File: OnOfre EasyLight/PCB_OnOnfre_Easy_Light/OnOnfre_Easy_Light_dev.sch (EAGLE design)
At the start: 27 parts, among them J3Y S8050, K1 OMRON-G3MB-202P-SSR2, K2 OMRON-G3MB-202P-SSR2, U2 esp12

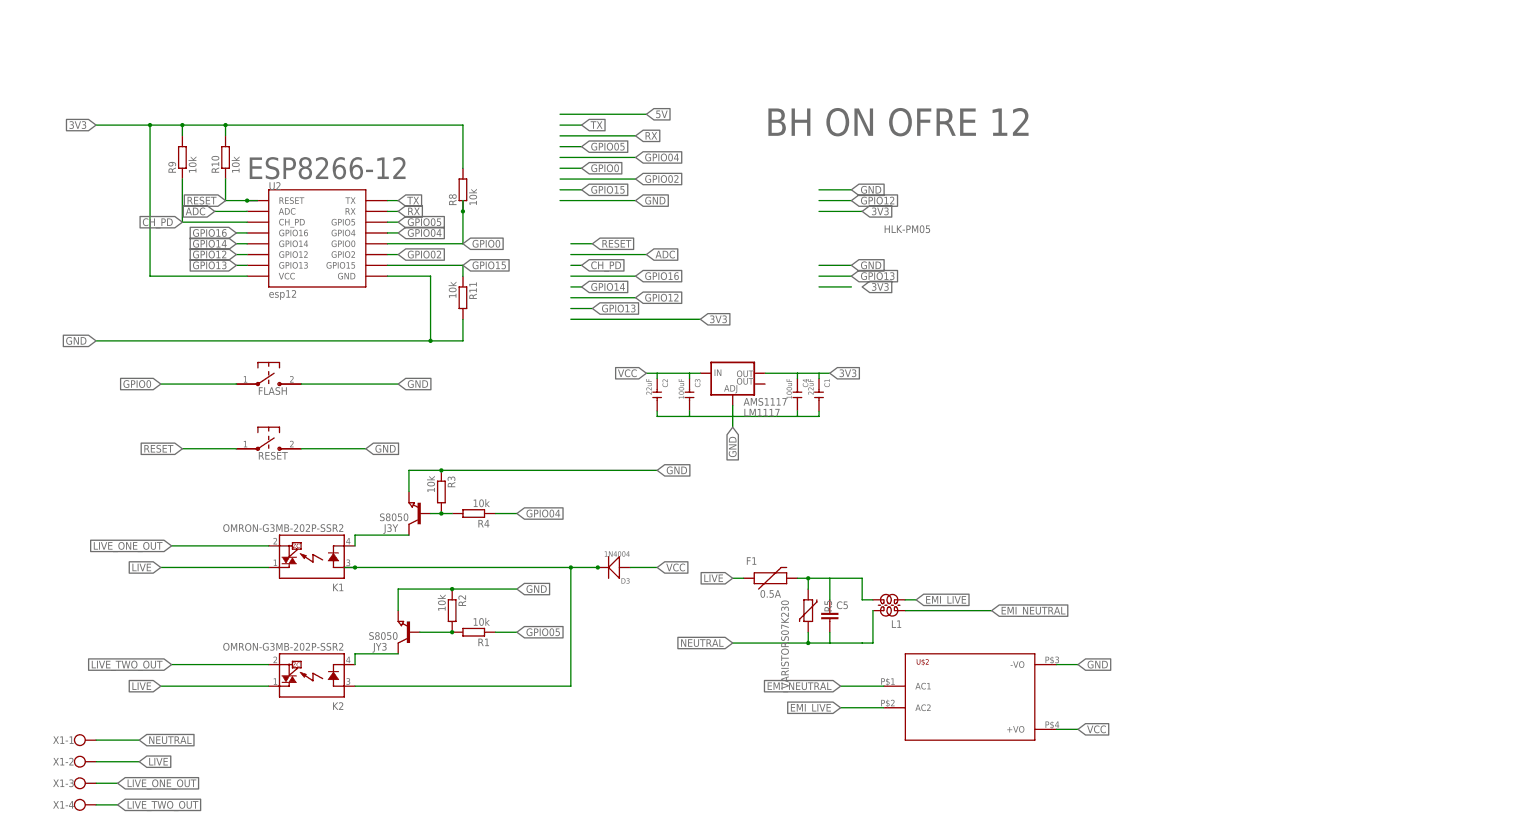
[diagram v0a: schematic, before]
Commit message: no message
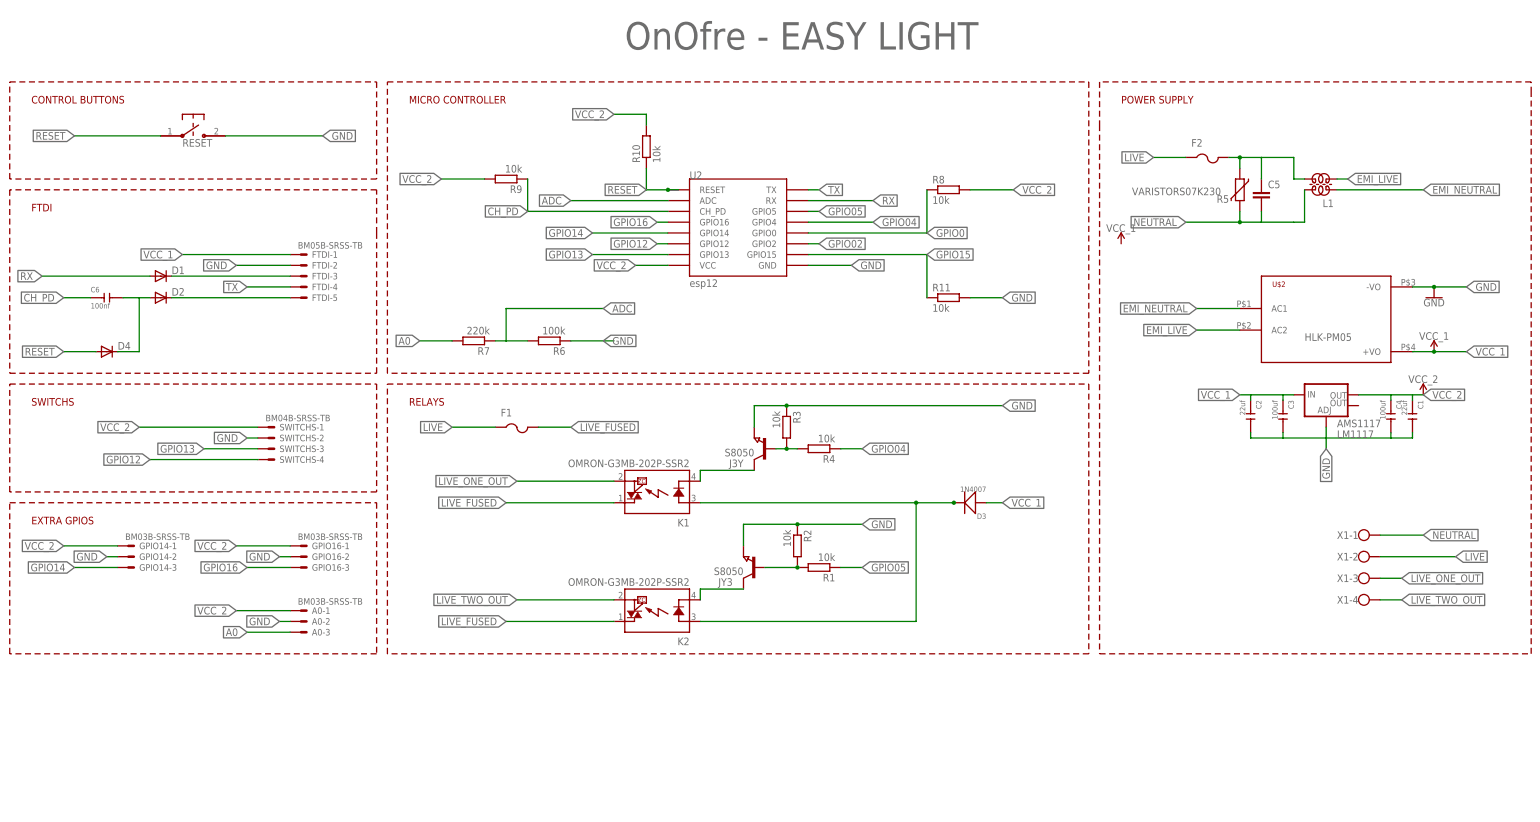
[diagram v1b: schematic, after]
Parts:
- removed FLASH: B3U-1000P-2P-SMD, switches:B3U-1000P
- added A0, GPIO14, GPIO16: BM03B-SRSS-TB, con-jst2:BM03B-SRSS-TB
- added C6: 100nf, Seeed-Capacitor:CERAMIC-100NF-50V-10%-X7R(0603)
- added D1, D2, D4: (no value), diode:DIODE-SOD323-R
- added F2: (no value), adafruit:PTCFUSE-1812
- added FTDI: BM05B-SRSS-TB, con-jst2:BM05B-SRSS-TB
- added R6: 100k, resistor:R-EU_R0603
- added R7: 220k, resistor:R-EU_R0603
- added SWITCHS: BM04B-SRSS-TB, con-jst2:BM04B-SRSS-TB
- C1, C2: value 22uF -> 22uf
- C3, C4: value 100uF -> 100uf
- D3: value 1N4004 -> 1N4007
- F1: value 0.5A -> (none); device SparkFun-Fuses:PPTC_PTH -> adafruit:PTCFUSE-1812
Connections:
- removed net 3V3: AMS1117.OUT, C1.1, C4.1, R10.2, R8.2, R9.2, U2.VCC
- removed net VCC: AMS1117.IN, C2.1, C3.1, D3.+, U$2.+VO
- new net A0: A0-3.S, R7.2
- new net DTR: D2.C, FTDI-5.S
- new net LIVE_FUSED: F1.2, K1.DS1, K2.DS1
- new net N$3: D1.C, FTDI-3.S
- new net N$4: C6.2, D2.A, D4.C
- new net VCC_1: AMS1117.IN, C2.1, C3.1, D3.+, FTDI-1.S, U$2.+VO
- new net VCC_2: A0-1.S, AMS1117.OUT, C1.1, C4.1, GPIO14-1.S, GPIO16-1.S, R10.2, R8.2, R9.2, SWITCHS-1.S, U2.VCC
- net ADC: now also R6.2, R7.1
- net CH_PD: now also C6.1
- net GND: now also A0-2.S, FTDI-2.S, GPIO14-2.S, GPIO16-2.S, R6.1, SWITCHS-2.S; no longer FLASH.P$2
- net GPIO0: no longer FLASH.P$1
- net GPIO12: now also SWITCHS-4.S
- net GPIO13: now also SWITCHS-3.S
- net GPIO14: now also GPIO14-3.S
- net GPIO16: now also GPIO16-3.S
- net LIVE: now also F2.1; no longer K1.DS1, K2.DS1
- net N$2: now also F2.2; no longer F1.2
- net RESET: now also D4.A
- net RX: now also D1.A
- net TX: now also FTDI-4.S
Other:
- note added: "CONTROL BUTTONS"
- note added: "EXTRA GPIOS"
- note added: "FTDI"
- note added: "MICRO CONTROLLER"
- note added: "OnOfre - EASY LIGHT"
- note added: "POWER SUPPLY"
- note added: "RELAYS"
- note added: "SWITCHS"
- note removed: "BH ON OFRE 12"
- note removed: "ESP8266-12"
- moved on the sheet: AMS1117, C1, C2, C3, C4, C5, D3, J3Y, JY3, K1, K2, L1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
